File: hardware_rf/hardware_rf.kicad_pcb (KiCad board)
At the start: 4 copper layers, 72 x 72 mm, 91 parts, among them IC1 CC1125RHBR, IC2 BALF-SPI2-02D3, IC3 4259-63, IC4 4259-63, J1 Conn_Coaxial, J3 Conn_02x20_Top_Bottom, J4 USB_C_Receptacle_USB2.0_16P, SW1 SW_Push, U1 RP2350A-QFN60, U2 W25Q128JVS, U3 GSQ5111, U4 SK5129, U5 AMS1117s-3.3, Y1 Crystal_GND24, Y2 Crystal_GND24

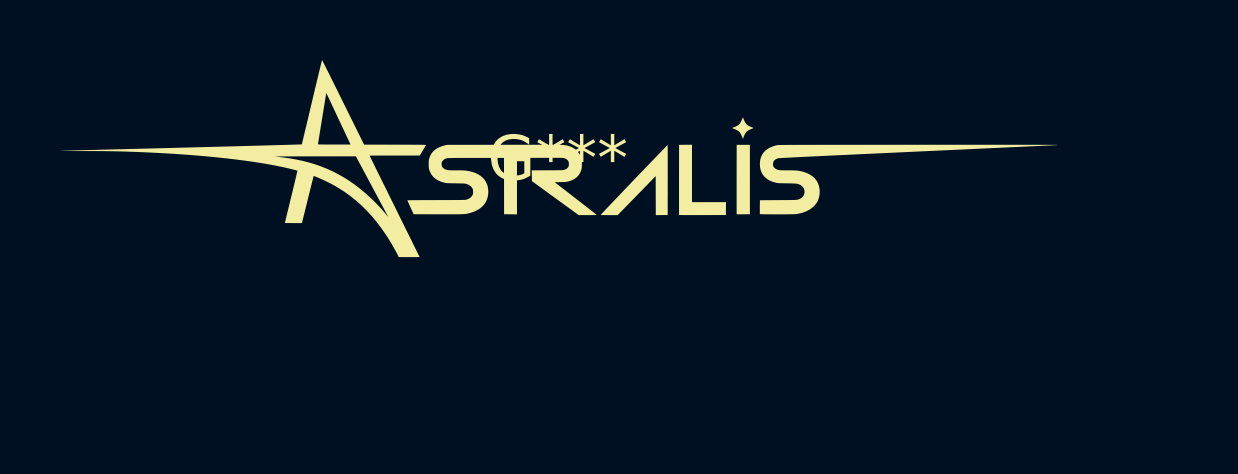
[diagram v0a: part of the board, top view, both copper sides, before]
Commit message: pcb
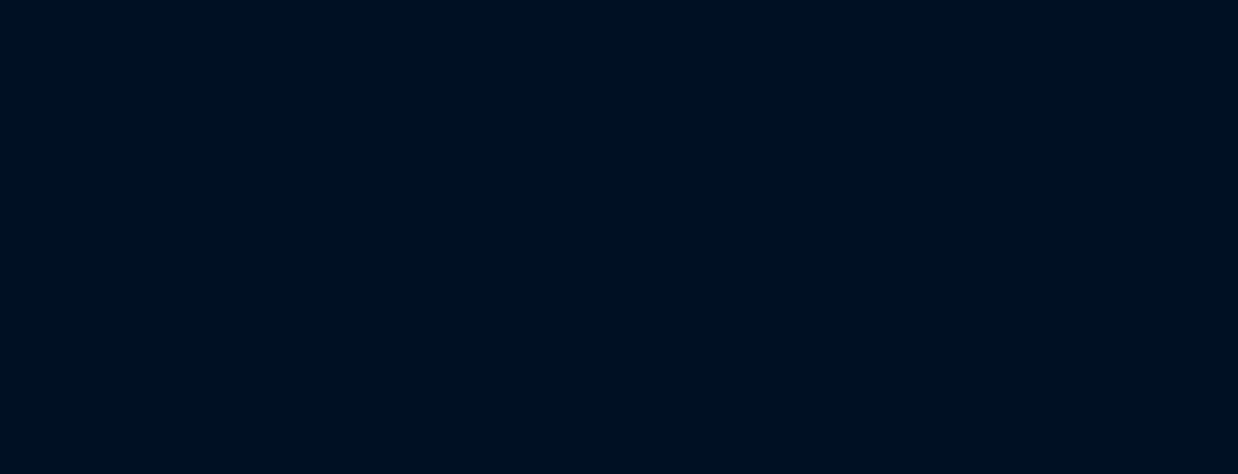
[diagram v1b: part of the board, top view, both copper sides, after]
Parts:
- removed the G*** at (0.00, 0.00)
